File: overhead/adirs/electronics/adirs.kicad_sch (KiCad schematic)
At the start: 61 parts, among them J1 Conn_02x01, J2 Conn_02x13_Counter_Clockwise, J3 Conn_02x01, J4 Conn_02x02_Counter_Clockwise, J5 Conn_02x02_Counter_Clockwise, J6 Conn_02x02_Counter_Clockwise

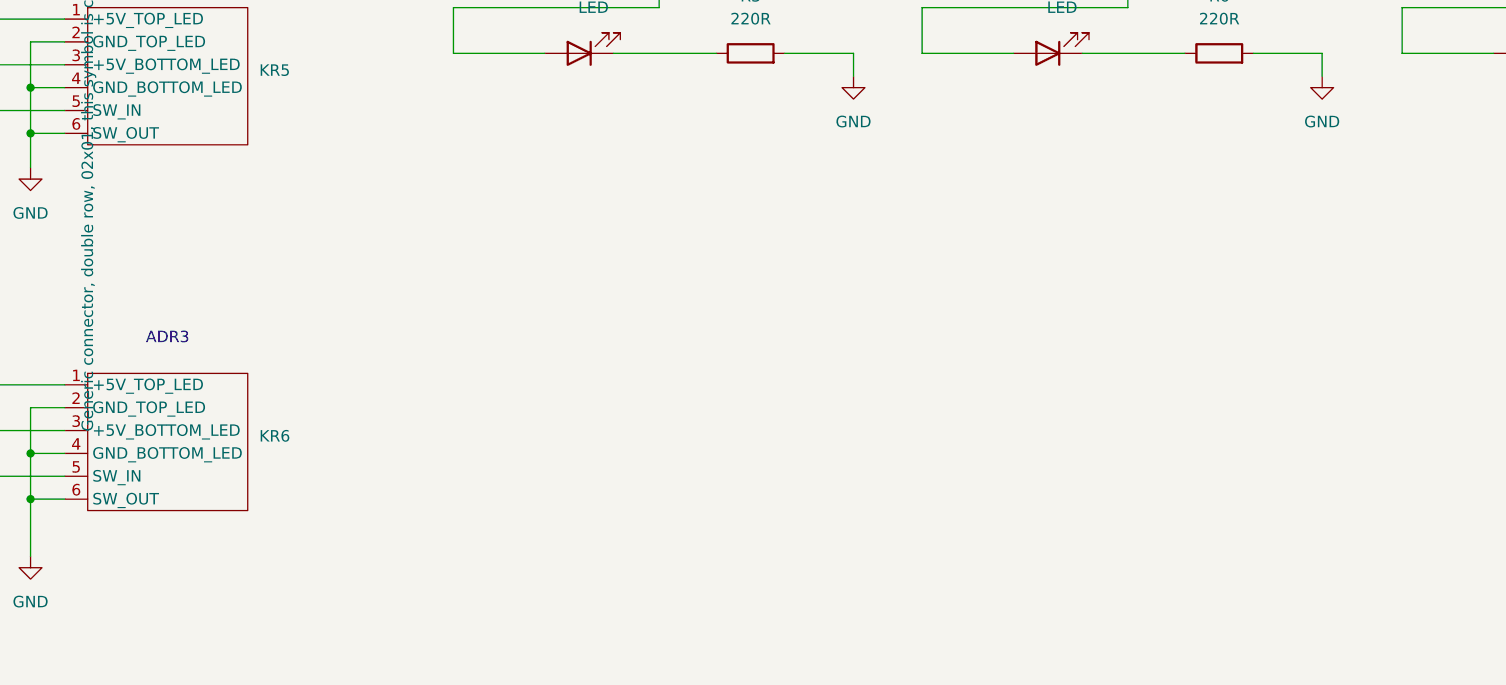
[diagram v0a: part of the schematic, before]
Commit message: Updates and Routing to ADIRS PCB and Schematic
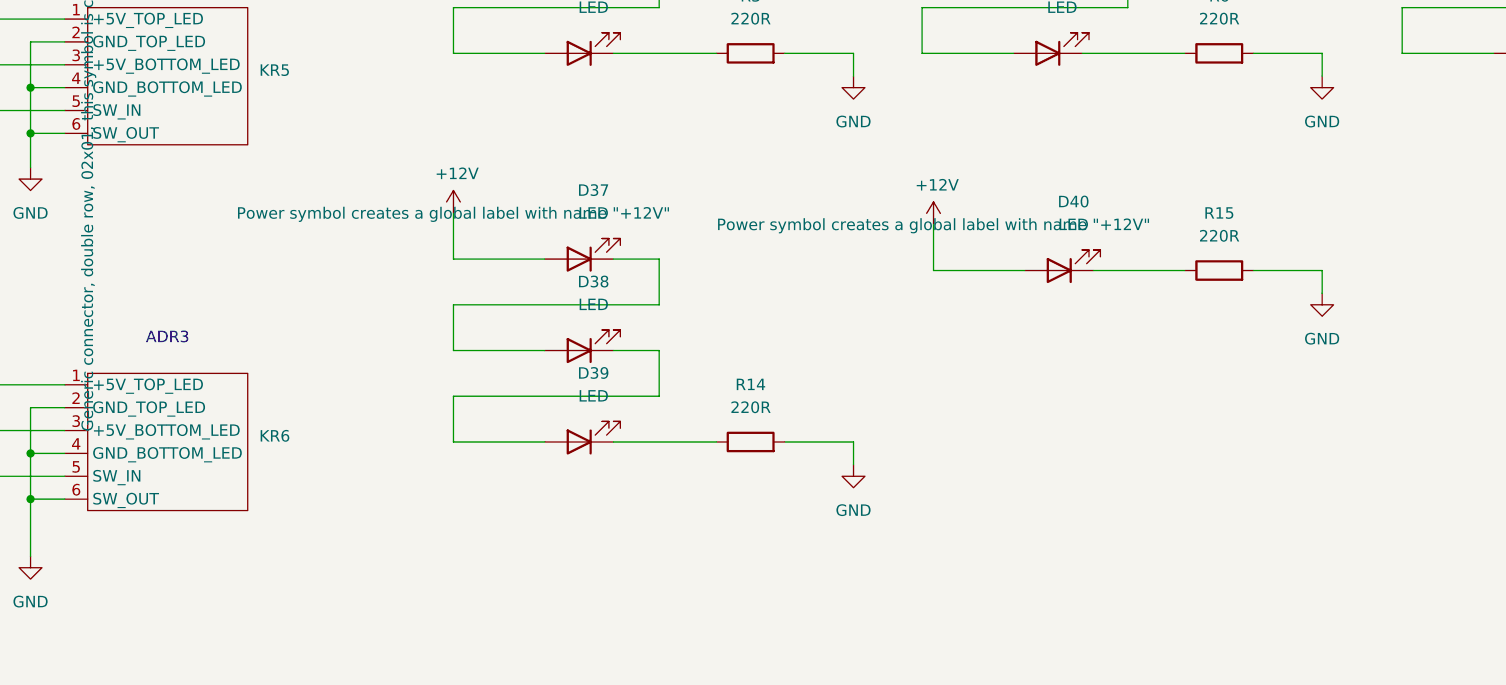
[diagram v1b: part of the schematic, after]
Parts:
- added D37, D38, D39, D40: LED, LED_THT:LED_D5.0mm, symbol Device:LED
- added R14, R15: 220R, Resistor_SMD:R_1206_3216Metric_Pad1.30x1.75mm_HandSolder, symbol Device:R
- J2: footprint TerminalBlock:TerminalBlock_bornier-2_P5.08mm -> Connector_PinHeader_2.54mm:PinHeader_2x14_P2.54mm_Vertical
- J3: footprint TerminalBlock:TerminalBlock_bornier-2_P5.08mm -> Connector_PinHeader_2.54mm:PinHeader_1x02_P2.54mm_Vertical
- J4, J5, J6: footprint TerminalBlock:TerminalBlock_bornier-2_P5.08mm -> TerminalBlock:TerminalBlock_bornier-4_P5.08mm
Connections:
- net +12V: now also D37.2 (A), D40.2 (A)
- net GND: now also R14.2, R15.2
- new net: D39.1 (K), R14.1
- new net: D40.1 (K), R15.1
- new net: D38.1 (K), D39.2 (A)
- new net: D37.1 (K), D38.2 (A)
